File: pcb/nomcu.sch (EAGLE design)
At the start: 36 parts, among them IC4 MY_7905DT, J1 ATX24RH

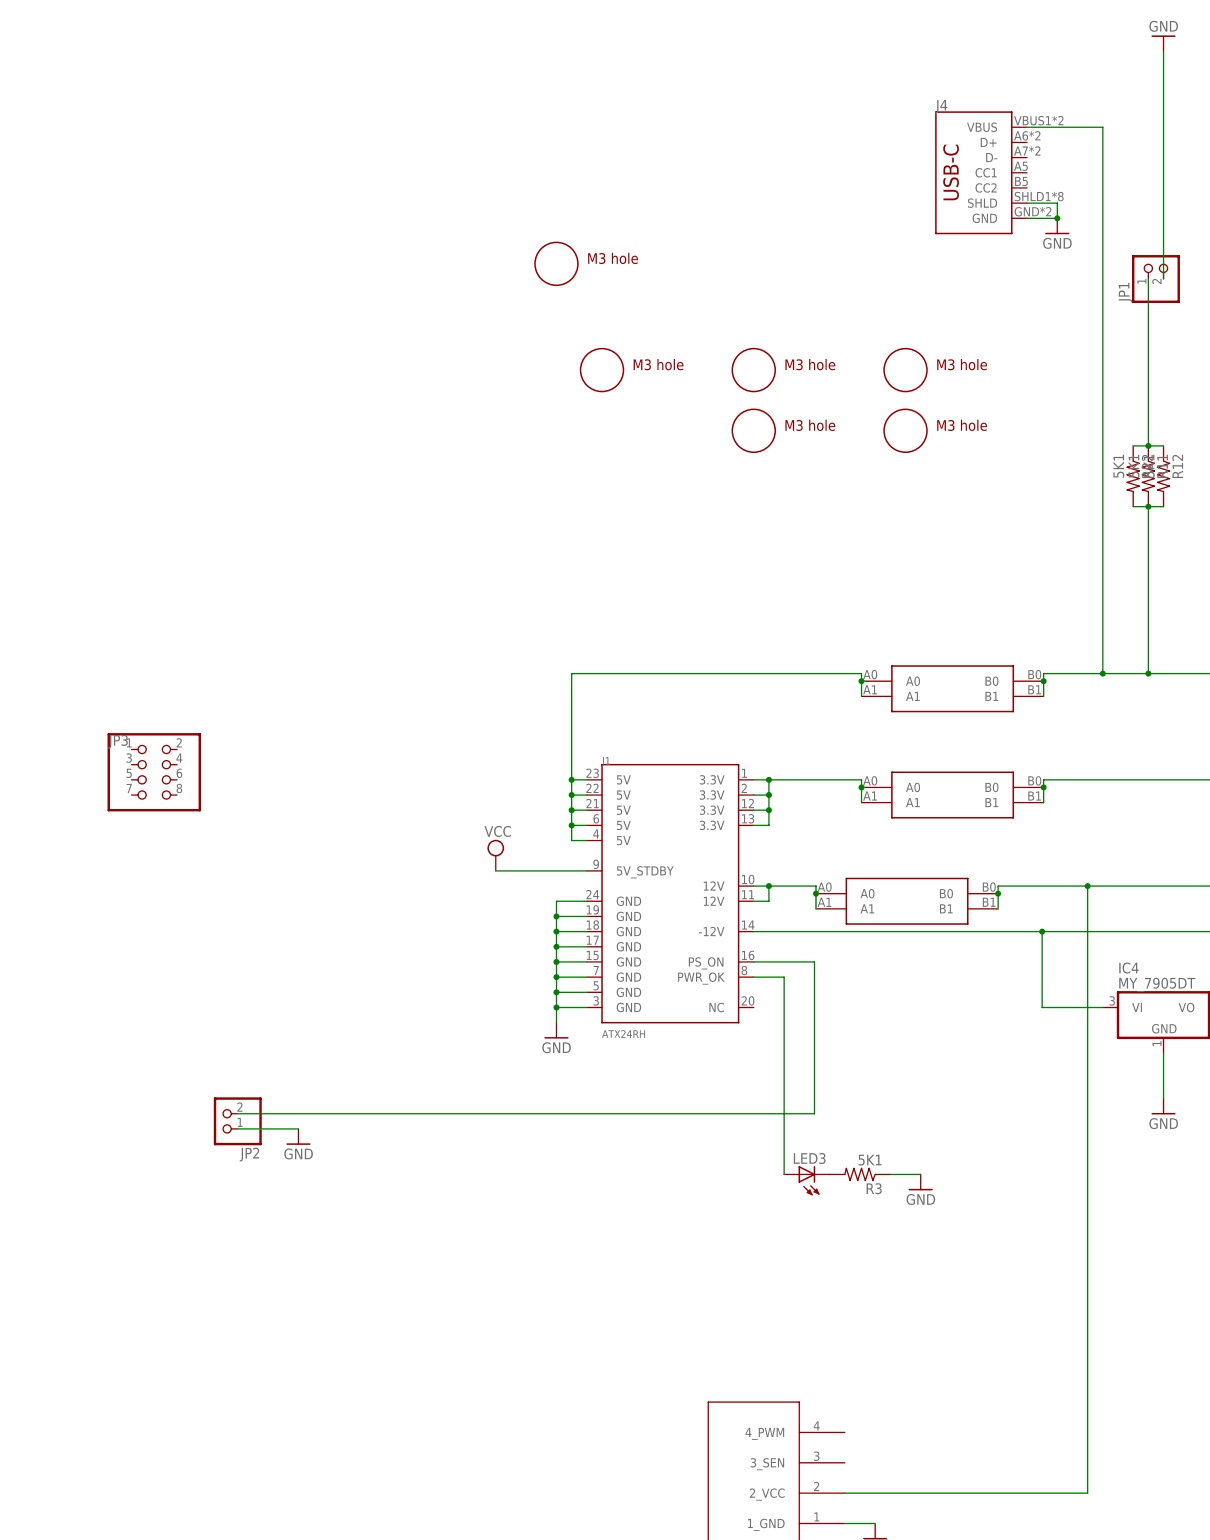
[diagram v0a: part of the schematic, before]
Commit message: working on new version
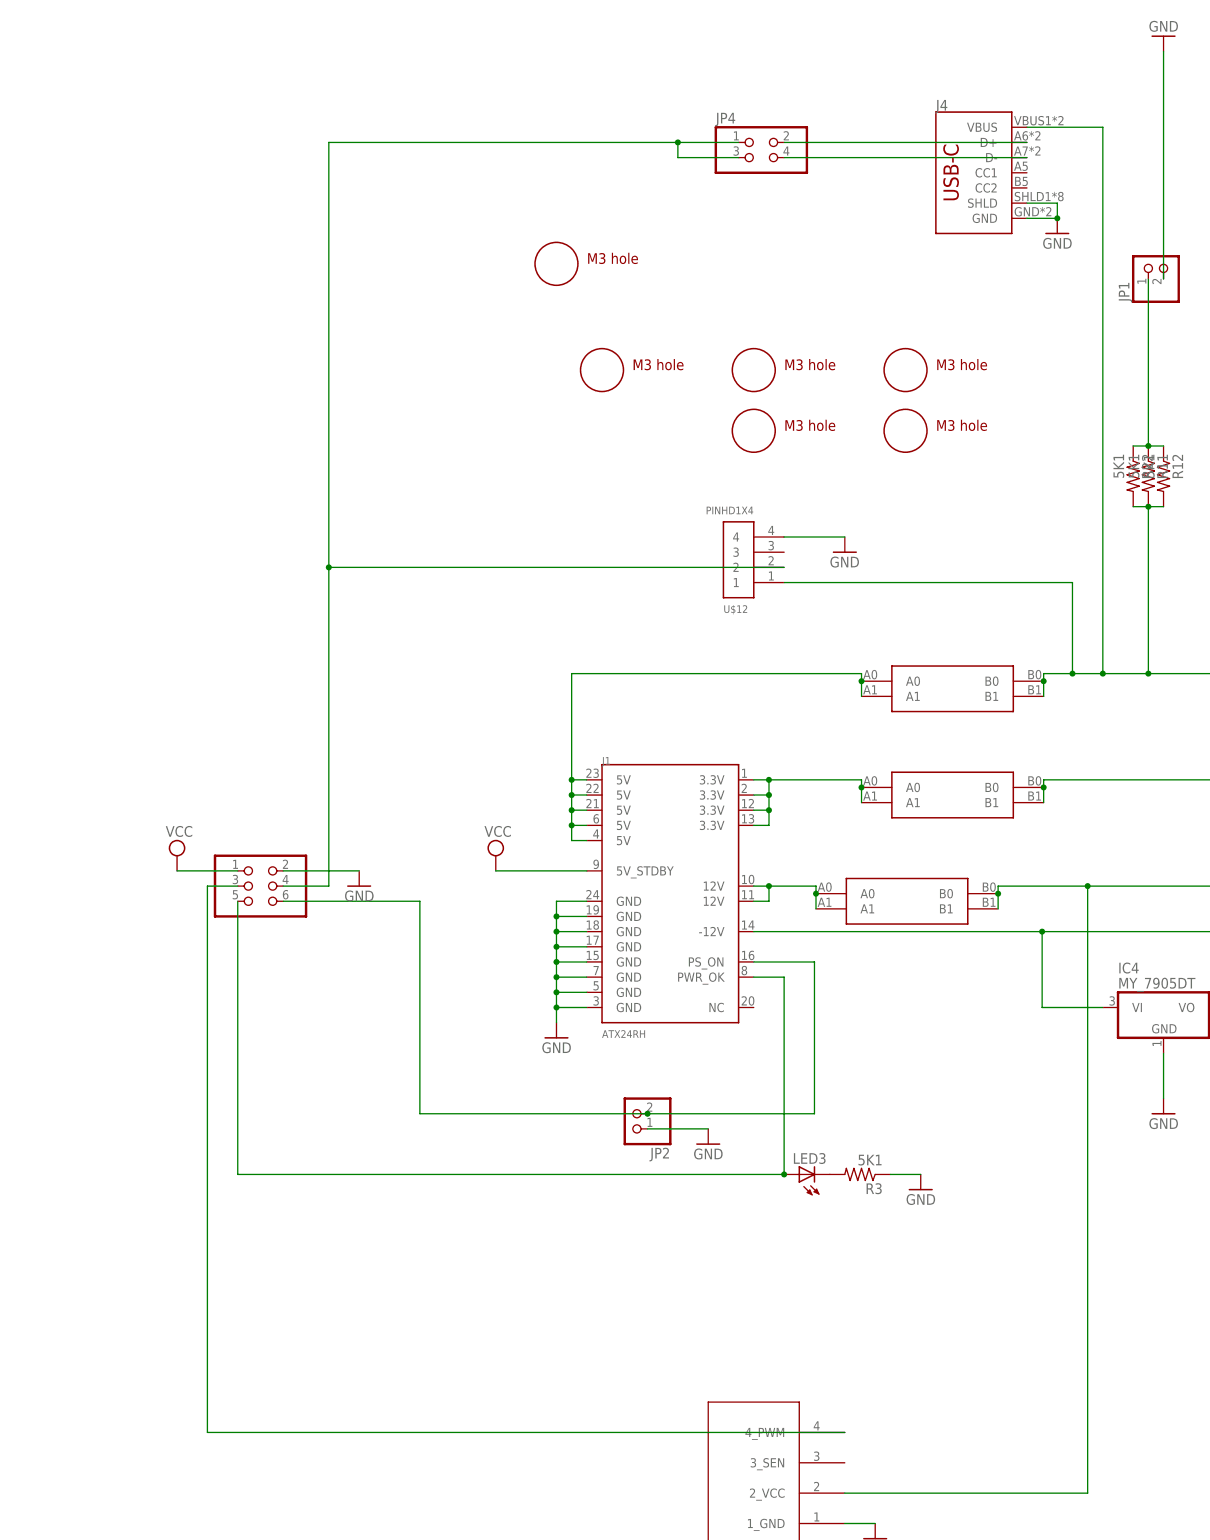
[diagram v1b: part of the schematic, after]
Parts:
- added JP4: (no value), pinhead:PINHD-2X2
- added U$12: PINHD1X4, adafruit_changed:PINHD1X4
- J1: device SparkFun-Connectors:ATX24RH -> nomcu:ATX24RH
- JP3: device pinhead:PINHD-2X4 -> pinhead:PINHD-2X3
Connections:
- new net N$3: JP3.3, JP8.4_PWM
- new net N$4: J4.D+, JP4.2
- new net N$6: J4.D-, JP4.4
- new net N$7: JP3.4, JP4.1, JP4.3, U$12.2
- net F5V: now also U$12.1
- net GND: now also JP3.2, U$12.4
- net N$11: now also JP3.5
- net N$15: now also JP3.6
- net VCC: now also JP3.1
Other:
- moved on the sheet: JP2
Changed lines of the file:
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@@
 <part name="U$2" library="a" deviceset="M3_MOUNTING_HOLE" device=""/>
 <part name="U$3" library="a" deviceset="M3_MOUNTING_HOLE" device=""/>
-<part name="J1" library="SparkFun-Connectors" deviceset="ATX24" device="RH"/>
+<part name="J1" library="nomcu" deviceset="ATX24" device="RH"/>
 <part name="GND2" library="supply1" deviceset="GND" device=""/>
 <part name="SUPPLY5" library="supply2" library_urn="urn:adsk.eagle:library:372" deviceset="VCC" device=""/>
@@
 <part name="GND26" library="supply1" deviceset="GND" device=""/>
 <part name="J4" library="SparkFun-Connectors" deviceset="USB_C" device="16PIN"/>
-<part name="JP3" library="pinhead" library_urn="urn:adsk.eagle:library:325" deviceset="PINHD-2X4" device="" package3d_urn="urn:adsk.eagle:package:22461/2"/>
+<part name="JP3" library="pinhead" library_urn="urn:adsk.eagle:library:325" deviceset="PINHD-2X3" device="" package3d_urn="urn:adsk.eagle:package:22462/2"/>
 <part name="U$6" library="a" deviceset="M3_MOUNTING_HOLE" device=""/>
 <part name="U$11" library="a" deviceset="M3_MOUNTING_HOLE" device=""/>
 <part name="JP2" library="pinhead" library_urn="urn:adsk.eagle:library:325" deviceset="PINHD-1X2" device="" package3d_urn="urn:adsk.eagle:package:22435/2"/>
+<part name="SUPPLY1" library="supply2" library_urn="urn:adsk.eagle:library:372" deviceset="VCC" device=""/>
+<part name="GND1" library="supply1" deviceset="GND" device=""/>
+<part name="GND3" library="backplane" deviceset="GND" device=""/>
+<part name="U$12" library="adafruit_changed" deviceset="PINHD1X4" device=""/>
+<part name="JP4" library="pinhead" library_urn="urn:adsk.eagle:library:325" deviceset="PINHD-2X2" device="" package3d_urn="urn:adsk.eagle:package:22455/2"/>
 </parts>
 <sheets>
@@
 <attribute name="VALUE" x="447.04" y="38.1" size="1.778" layer="96"/>
 </instance>
-<instance part="GND24" gate="1" x="172.72" y="-38.1" smashed="yes" rot="MR0">
-<attribute name="VALUE" x="175.26" y="-40.64" size="1.778" layer="96" rot="MR0"/>
+<instance part="GND24" gate="1" x="241.3" y="-38.1" smashed="yes" rot="MR0">
+<attribute name="VALUE" x="243.84" y="-40.64" size="1.778" layer="96" rot="MR0"/>
 </instance>
 <instance part="GND32" gate="1" x="276.86" y="-45.72" smashed="yes" rot="MR0">
@@
 <attribute name="NAME" x="279.4" y="134.874" size="1.778" layer="95" font="vector"/>
 </instance>
-<instance part="JP3" gate="A" x="147.32" y="22.86" smashed="yes">
-<attribute name="NAME" x="140.97" y="28.575" size="1.778" layer="95"/>
-<attribute name="VALUE" x="140.97" y="15.24" size="1.778" layer="96"/>
+<instance part="JP3" gate="A" x="165.1" y="5.08" smashed="yes">
+<attribute name="VALUE" x="158.75" y="-2.54" size="1.778" layer="96"/>
 </instance>
 <instance part="U$6" gate="G$1" x="223.52" y="91.44" smashed="yes"/>
 <instance part="U$11" gate="G$1" x="215.9" y="109.22" smashed="yes"/>
-<instance part="JP2" gate="G$1" x="160.02" y="-33.02" smashed="yes" rot="R180">
-<attribute name="NAME" x="166.37" y="-38.735" size="1.778" layer="95" rot="R180"/>
-<attribute name="VALUE" x="166.37" y="-27.94" size="1.778" layer="96" rot="R180"/>
+<instance part="JP2" gate="G$1" x="228.6" y="-33.02" smashed="yes" rot="R180">
+<attribute name="NAME" x="234.95" y="-38.735" size="1.778" layer="95" rot="R180"/>
+<attribute name="VALUE" x="234.95" y="-27.94" size="1.778" layer="96" rot="R180"/>
+</instance>
+<instance part="SUPPLY1" gate="G$1" x="152.4" y="10.16" smashed="yes">
+<attribute name="VALUE" x="150.495" y="13.335" size="1.778" layer="96"/>
+</instance>
+<instance part="GND1" gate="1" x="182.88" y="5.08" smashed="yes" rot="MR0">
+<attribute name="VALUE" x="185.42" y="2.54" size="1.778" layer="96" rot="MR0"/>
+</instance>
+<instance part="GND3" gate="1" x="264.16" y="60.96" smashed="yes">
+<attribute name="VALUE" x="261.62" y="58.42" size="1.778" layer="96"/>
+</instance>
+<instance part="U$12" gate="1" x="248.92" y="58.42" smashed="yes" rot="R180">
+<attribute name="NAME" x="243.84" y="50.8" size="1.27" layer="95" font="vector"/>
+<attribute name="VALUE" x="248.92" y="68.58" size="1.27" layer="96" font="vector" rot="R180"/>
+</instance>
+<instance part="JP4" gate="A" x="251.46" y="127" smashed="yes">
+<attribute name="NAME" x="242.57" y="132.715" size="1.778" layer="95"/>
+<attribute name="VALUE" x="242.57" y="121.92" size="1.778" layer="96"/>
 </instance>
 </instances>
@@
 <pinref part="GND24" gate="1" pin="GND"/>
 <pinref part="JP2" gate="G$1" pin="1"/>
-<wire x1="172.72" y1="-35.56" x2="162.56" y2="-35.56" width="0.1524" layer="91"/>
+<wire x1="241.3" y1="-35.56" x2="231.14" y2="-35.56" width="0.1524" layer="91"/>
+</segment>
+<segment>
+<pinref part="GND1" gate="1" pin="GND"/>
+<pinref part="JP3" gate="A" pin="2"/>
+<wire x1="182.88" y1="7.62" x2="170.18" y2="7.62" width="0.1524" layer="91"/>
+</segment>
+<segment>
+<pinref part="U$12" gate="1" pin="4"/>
+<pinref part="GND3" gate="1" pin="GND"/>
+<wire x1="254" y1="63.5" x2="264.16" y2="63.5" width="0.1524" layer="91"/>
 </segment>
 </net>
@@
 <pinref part="SUPPLY6" gate="G$1" pin="VCC"/>
 <wire x1="220.98" y1="7.62" x2="205.74" y2="7.62" width="0.1524" layer="91"/>
+</segment>
+<segment>
+<pinref part="SUPPLY1" gate="G$1" pin="VCC"/>
+<pinref part="JP3" gate="A" pin="1"/>
+<wire x1="152.4" y1="7.62" x2="162.56" y2="7.62" width="0.1524" layer="91"/>
 </segment>
 </net>
@@
 <junction x="314.96" y="40.64"/>
 <pinref part="U$8" gate="G$1" pin="B0"/>
-<wire x1="307.34" y1="40.64" x2="297.434" y2="40.64" width="0.1524" layer="91"/>
 <wire x1="297.434" y1="40.64" x2="297.434" y2="39.37" width="0.1524" layer="91"/>
 <junction x="307.34" y="40.64"/>
@@
 <pinref part="U$9" gate="G$1" pin="P$4"/>
 <wire x1="388.62" y1="-43.18" x2="381" y2="-43.18" width="0.1524" layer="91"/>
+<wire x1="307.34" y1="40.64" x2="302.26" y2="40.64" width="0.1524" layer="91"/>
+<wire x1="302.26" y1="40.64" x2="297.434" y2="40.64" width="0.1524" layer="91"/>
+<wire x1="254" y1="55.88" x2="302.26" y2="55.88" width="0.1524" layer="91"/>
+<wire x1="302.26" y1="55.88" x2="302.26" y2="40.64" width="0.1524" layer="91"/>
+<junction x="302.26" y="40.64"/>
+<pinref part="U$12" gate="1" pin="1"/>
 </segment>
 </net>
@@
 <wire x1="254" y1="-10.16" x2="254" y2="-43.18" width="0.1524" layer="91"/>
 <pinref part="LED3" gate="G$1" pin="A"/>
+<pinref part="JP3" gate="A" pin="5"/>
+<wire x1="254" y1="-43.18" x2="162.56" y2="-43.18" width="0.1524" layer="91"/>
+<wire x1="162.56" y1="-43.18" x2="162.56" y2="2.54" width="0.1524" layer="91"/>
+<junction x="254" y="-43.18"/>
 </segment>
 </net>
@@
 <wire x1="259.08" y1="-7.62" x2="248.92" y2="-7.62" width="0.1524" layer="91"/>
 <wire x1="259.08" y1="-33.02" x2="259.08" y2="-7.62" width="0.1524" layer="91"/>
-<wire x1="259.08" y1="-33.02" x2="162.56" y2="-33.02" width="0.1524" layer="91"/>
+<wire x1="259.08" y1="-33.02" x2="231.14" y2="-33.02" width="0.1524" layer="91"/>
 <pinref part="JP2" gate="G$1" pin="2"/>
-</segment>
-</net>
+<wire x1="193.04" y1="2.54" x2="193.04" y2="-33.02" width="0.1524" layer="91"/>
+<wire x1="193.04" y1="-33.02" x2="231.14" y2="-33.02" width="0.1524" layer="91"/>
+<junction x="231.14" y="-33.02"/>
+<pinref part="JP3" gate="A" pin="6"/>
+<wire x1="193.04" y1="2.54" x2="170.18" y2="2.54" width="0.1524" layer="91"/>
+</segment>
+</net>
+<net name="N$3" class="0">
+<segment>
+<pinref part="JP3" gate="A" pin="3"/>
+<wire x1="162.56" y1="5.08" x2="157.48" y2="5.08" width="0.1524" layer="91"/>
+<wire x1="157.48" y1="5.08" x2="157.48" y2="-86.36" width="0.1524" layer="91"/>
+<pinref part="JP8" gate="A" pin="4_PWM"/>
+<wire x1="157.48" y1="-86.36" x2="264.16" y2="-86.36" width="0.1524" layer="91"/>
+</segment>
+</net>
+<net name="N$4" class="0">
+<segment>
+<pinref part="J4" gate="J1" pin="D+"/>
+<wire x1="294.64" y1="129.54" x2="254" y2="129.54" width="0.1524" layer="91"/>
+<pinref part="JP4" gate="A" pin="2"/>
+</segment>
+</net>
+<net name="N$6" class="0">
+<segment>
+<pinref part="J4" gate="J1" pin="D-"/>
+<wire x1="294.64" y1="127" x2="254" y2="127" width="0.1524" layer="91"/>
+<pinref part="JP4" gate="A" pin="4"/>
+</segment>
+</net>
+<net name="N$7" class="0">
+<segment>
+<pinref part="JP4" gate="A" pin="1"/>
+<wire x1="246.38" y1="129.54" x2="236.22" y2="129.54" width="0.1524" layer="91"/>
+<wire x1="236.22" y1="129.54" x2="236.22" y2="127" width="0.1524" layer="91"/>
+<pinref part="JP4" gate="A" pin="3"/>
+<wire x1="236.22" y1="127" x2="246.38" y2="127" width="0.1524" layer="91"/>
+<pinref part="JP3" gate="A" pin="4"/>
+<wire x1="177.8" y1="5.08" x2="170.18" y2="5.08" width="0.1524" layer="91"/>
+<pinref part="U$12" gate="1" pin="2"/>
+<wire x1="177.8" y1="5.08" x2="177.8" y2="58.42" width="0.1524" layer="91"/>
+<wire x1="177.8" y1="58.42" x2="254" y2="58.42" width="0.1524" layer="91"/>
+<wire x1="236.22" y1="129.54" x2="177.8" y2="129.54" width="0.1524" layer="91"/>
+<wire x1="177.8" y1="129.54" x2="177.8" y2="58.42" width="0.1524" layer="91"/>
+<junction x="236.22" y="129.54"/>
+<junction x="177.8" y="58.42"/>
+</segment>
+</net>
